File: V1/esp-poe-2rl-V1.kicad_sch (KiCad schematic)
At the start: 56 parts, among them J1 USB_C_Receptacle_USB2.0, J2 RJ45 JACK, J3 1x2P 5,08mm, J4 1x2P 5,08mm, K1 G5NB-1A-E-DC5, K2 G5NB-1A-E-DC5, Q1 UMH3N, Q2 WPM2015-3/TR, Q3 LMUN2211LT1G, Q4 MMBT2222A, Q5 MMBT2222A, SW1 RESET, U4 CH340C, U5 ESP32-WROOM-32UE-N16, U6 LAN8710A

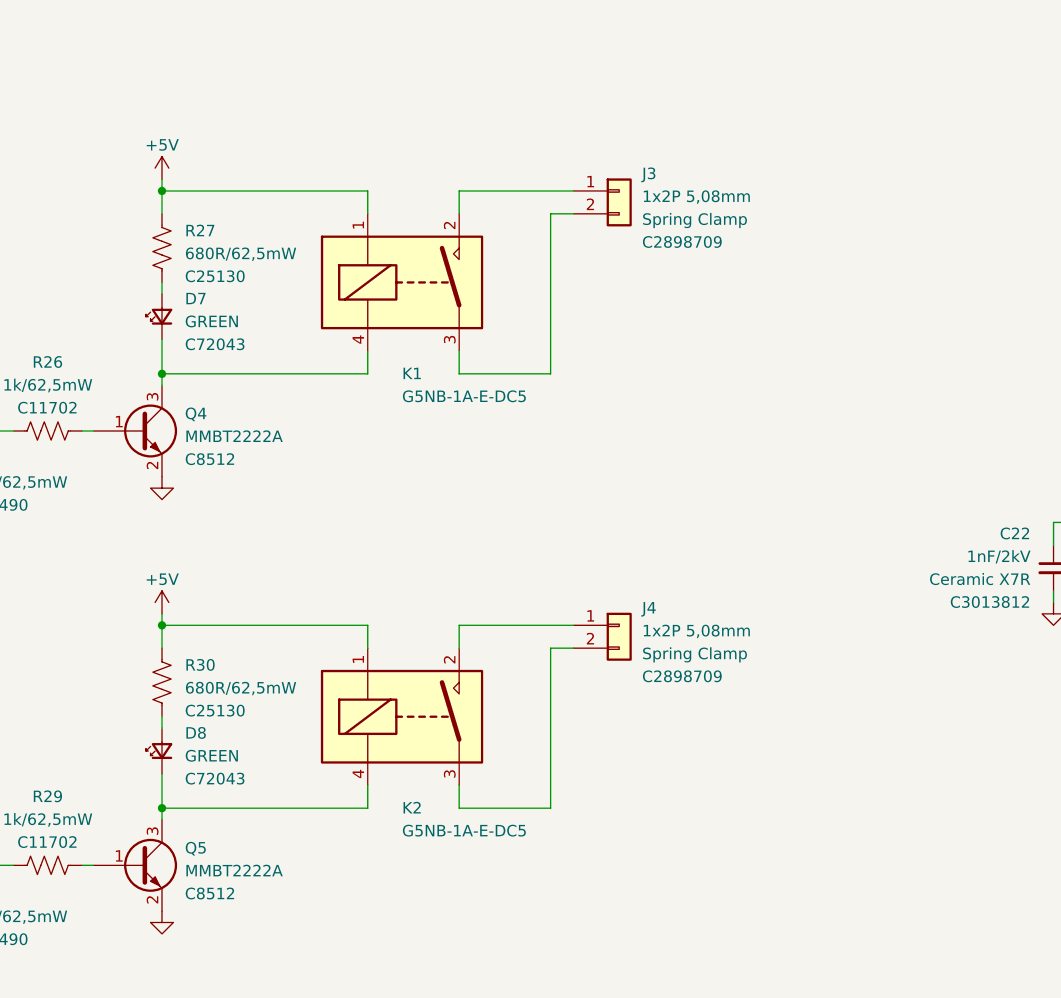
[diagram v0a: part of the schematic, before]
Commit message: Tweaks to components
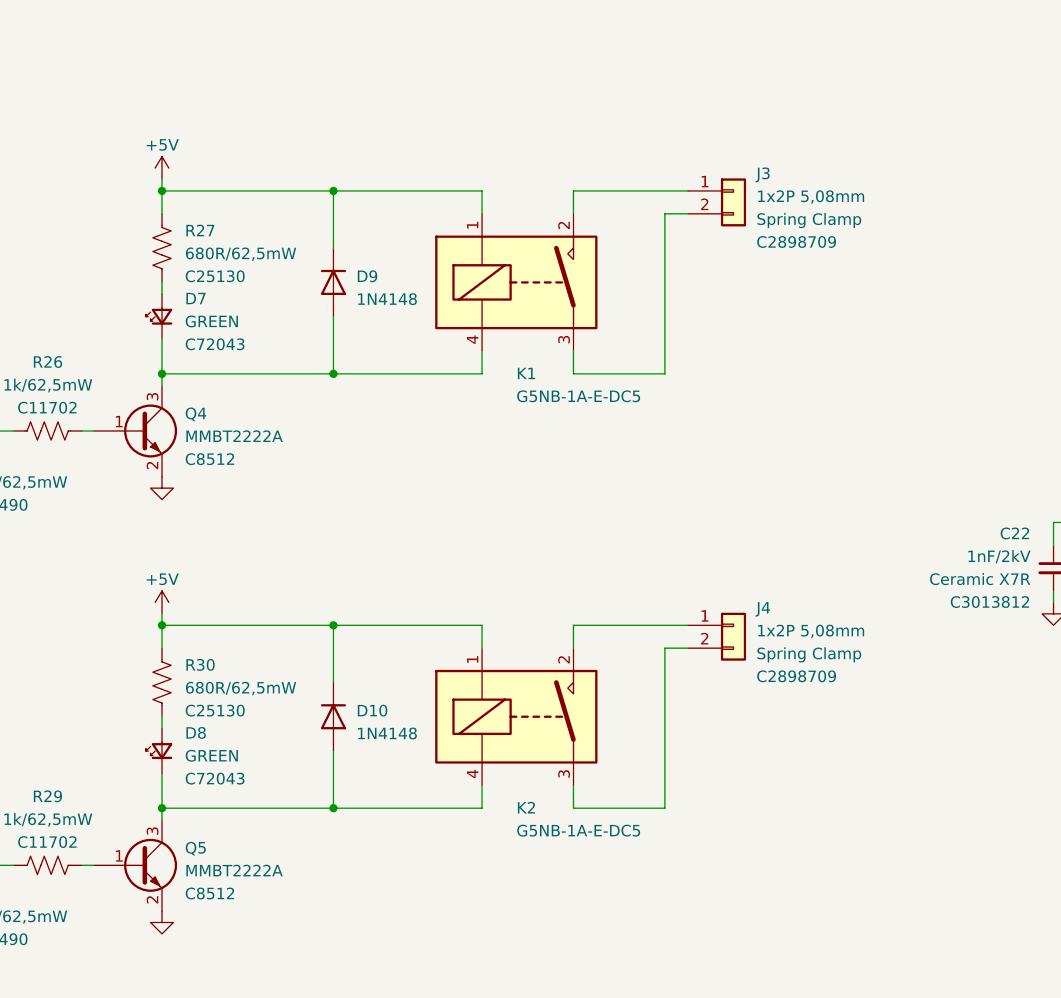
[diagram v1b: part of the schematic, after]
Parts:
- added D10, D9: 1N4148, Tales:D_SOD-123, symbol Diode:1N4148
- C10, C11, C13, C14, C16, C17, C18, C20, C21, C23, R14, R15, R16, R17, R18, R19, R20, R21, R22, R23, R24, R25, R26, R27, R28, R29, R30: Case 0402/1005 -> (none); Package (none) -> 0402/1005
- C12, C15, C19, C25: Case 0603/1608 -> (none); Package (none) -> 0603/1608
- C22, C24: Case 1206/3216 -> (none); Package (none) -> 1206/3216
- D6: Case SOT-23-5 -> (none); Package (none) -> SOT-23-5
- D7, D8: Case 0603 -> (none); Package (none) -> 0603
- F1: Case 1206 -> (none); Package (none) -> 1206
- L3: Case 0805/2012 -> (none); Package (none) -> 0805/2012
- Q1: Case SOT-363 -> (none); Package (none) -> SOT-363
- Q2, Q3, Q4, Q5: Case SOT-23-3 -> (none); Package (none) -> SOT-23-3
- RN1, RN2, RN3: Case 4x0402 -> (none); Package (none) -> 4x0402
- SW1: Case SPST -> (none); Package (none) -> SPST
- U4: Case SOIC-16 -> (none); Package (none) -> SOIC-16
- U5: Case ESP32-WROOM-U -> (none); Package (none) -> ESP32-WROOM-U
- U6: Case QFN-32 -> (none); Package (none) -> QFN-32
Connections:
- net +5V: now also D10.1 (K), D9.1 (K)
- net at D8.1 (K), K2.4, Q5.3 (C): now also D10.2 (A)
- net at D7.1 (K), K1.4, Q4.3 (C): now also D9.2 (A)
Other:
- moved on the sheet: J3, J4, K1, K2

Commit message: Update image
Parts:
- J3, J4: footprint Tales:TerminalBlock_Dibo_DB142R-2-5.08_1x02_P5.08mm_Horizontal -> Tales:TerminalBlock_Dibo_DB142R-5.08-2P_1x02_P5.08mm_Horizontal
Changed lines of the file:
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@@
       (effects (font (size 1.27 1.27)) (justify left))
     )
-    (property "Footprint" "Tales:TerminalBlock_Dibo_DB142R-2-5.08_1x02_P5.08mm_Horizontal" (at 215.9 232.41 0)
+    (property "Footprint" "Tales:TerminalBlock_Dibo_DB142R-5.08-2P_1x02_P5.08mm_Horizontal" (at 215.9 232.41 0)
       (effects (font (size 1.27 1.27)) hide)
     )
@@
       (effects (font (size 1.27 1.27)) (justify left))
     )
-    (property "Footprint" "Tales:TerminalBlock_Dibo_DB142R-2-5.08_1x02_P5.08mm_Horizontal" (at 215.9 184.15 0)
-      (effects (font (size 1.27 1.27)) hide)
-    )
+    (property "Footprint" "Tales:TerminalBlock_Dibo_DB142R-5.08-2P_1x02_P5.08mm_Horizontal" (at 215.9 184.15 0)
+      (effects (font (size 1.27 1.27)) hide)
+    )
